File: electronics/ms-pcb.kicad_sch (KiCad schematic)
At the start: 27 parts, among them J1 Left motor, J2 Right motor, J3 XT60-M, U1 ESP32-S3-DEVKITC-1U-N8R2, U2 GY-521

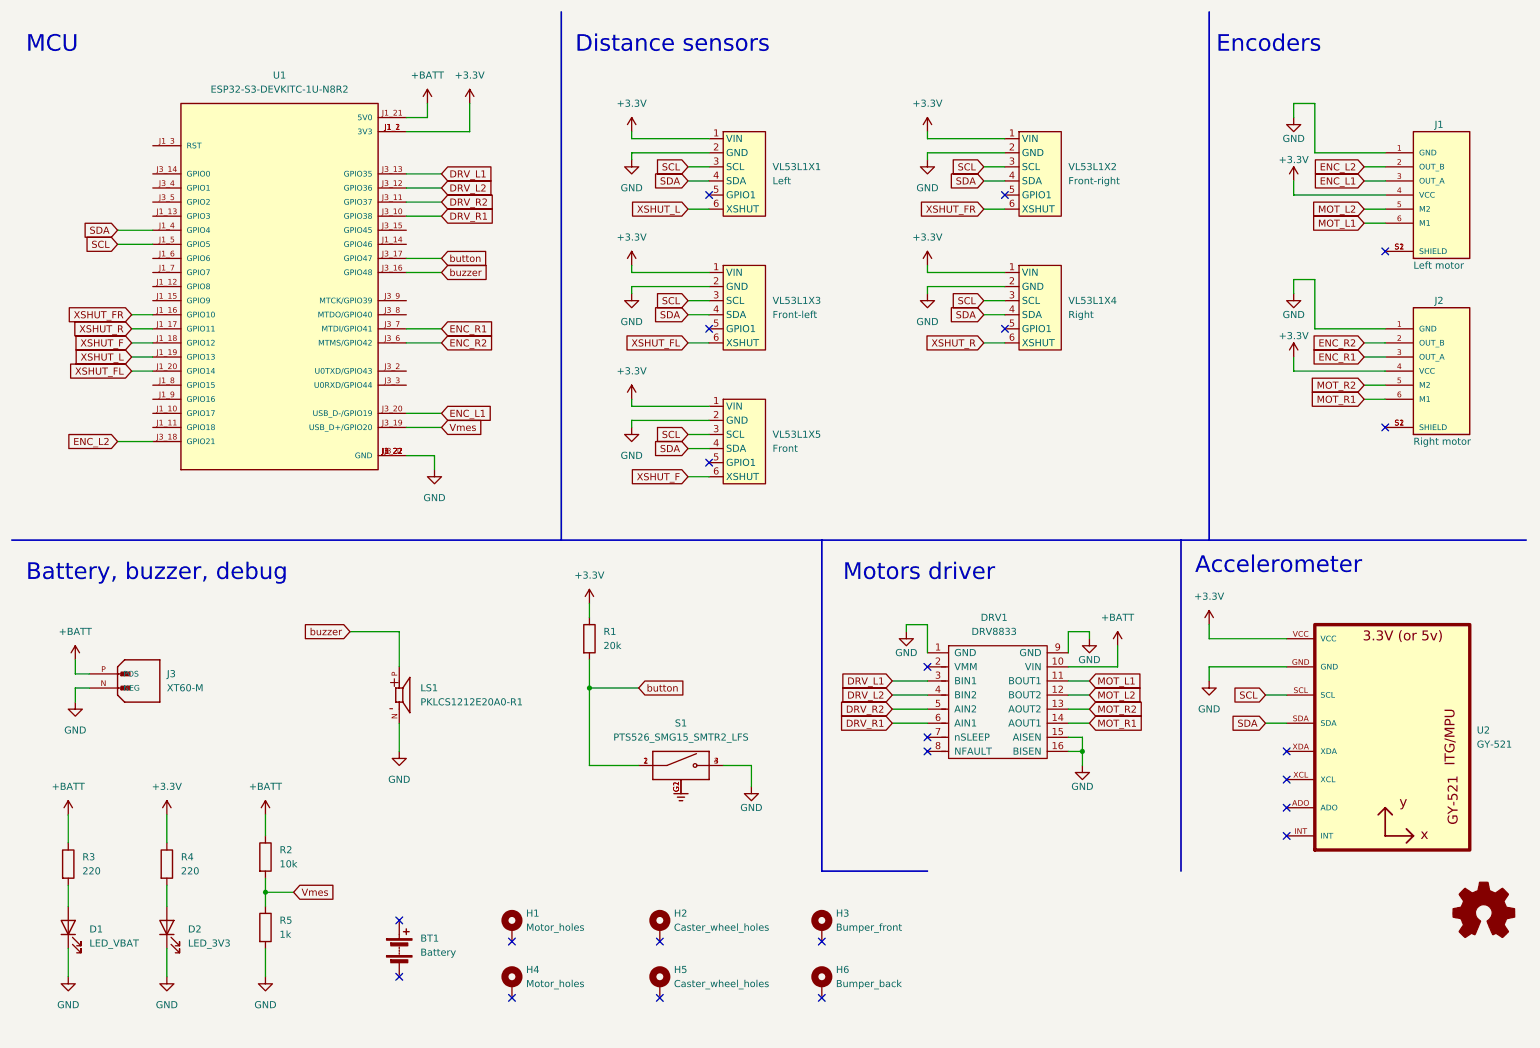
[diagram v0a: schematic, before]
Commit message: elec: start PCB v1.1.0
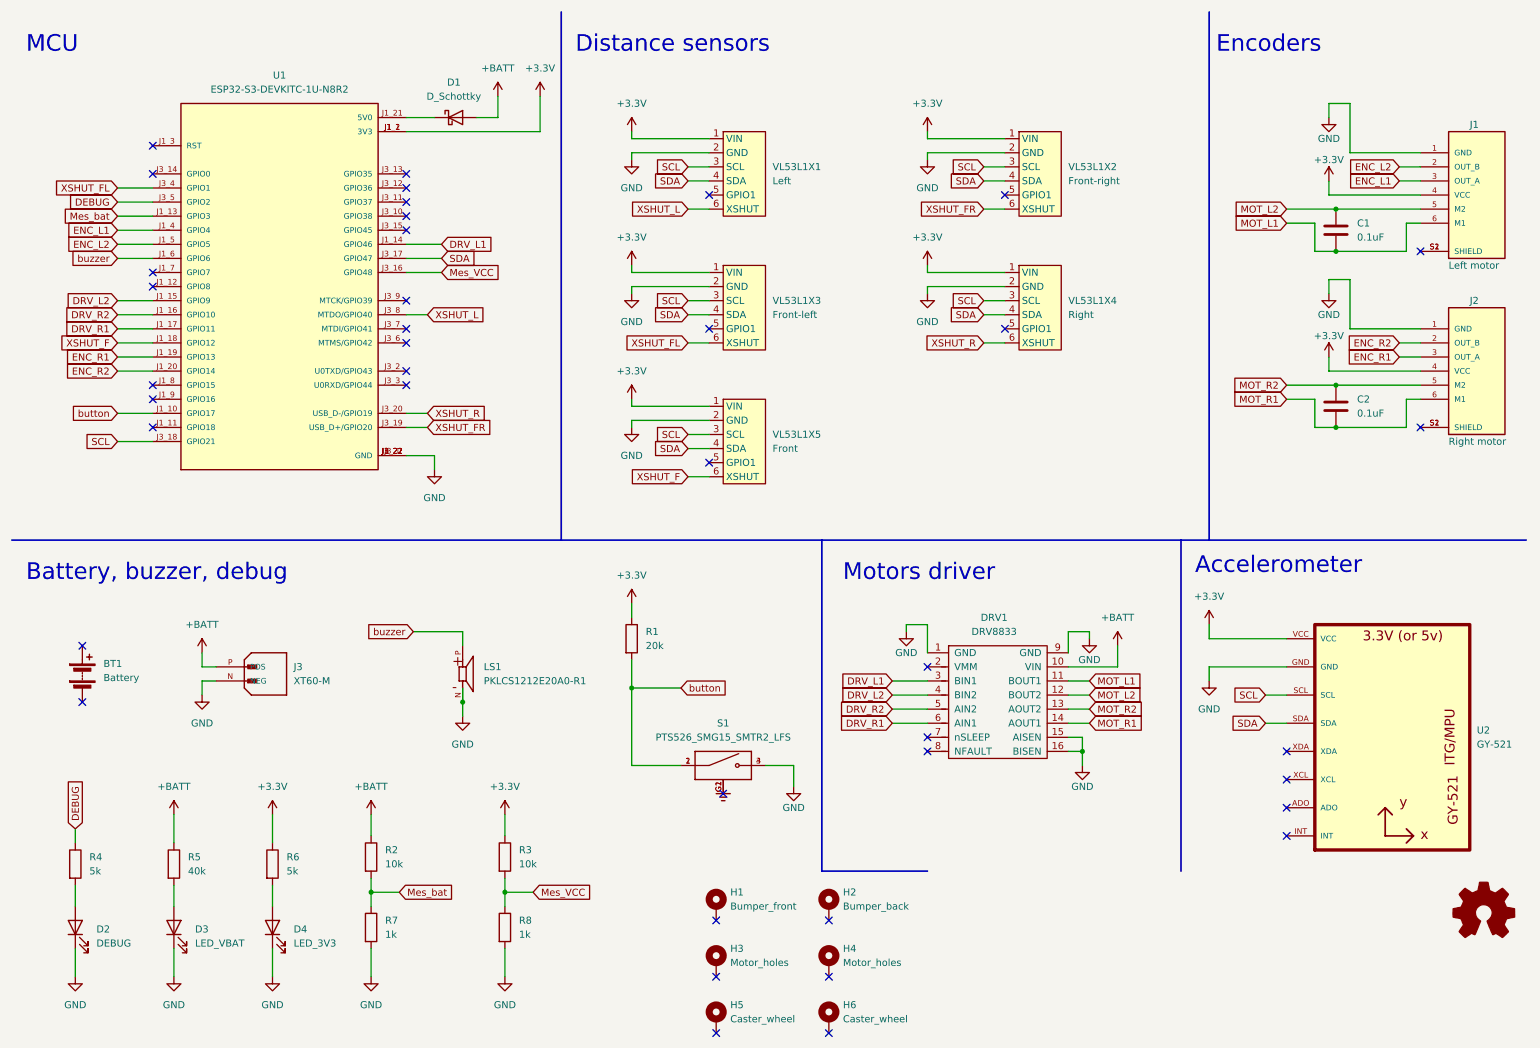
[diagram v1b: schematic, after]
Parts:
- added C1, C2: 0.1uF, Capacitor_THT:CP_Radial_D5.0mm_P2.00mm, symbol Device:C
- added D1: D_Schottky, Diode_SMD:D_1206_3216Metric_Pad1.42x1.75mm_HandSolder, symbol Device:D_Schottky
- added D2: DEBUG, LED_SMD:LED_1206_3216Metric_Pad1.42x1.75mm_HandSolder, symbol Device:LED
- added R3: 10k, Resistor_SMD:R_1206_3216Metric_Pad1.30x1.75mm_HandSolder, symbol Device:R
- added R4: 5k, Resistor_SMD:R_1206_3216Metric_Pad1.30x1.75mm_HandSolder, symbol Device:R
- added R8: 1k, Resistor_SMD:R_1206_3216Metric_Pad1.30x1.75mm_HandSolder, symbol Device:R
- H5: renamed from H2; value Caster_wheel_holes -> Caster_wheel
- H6: renamed from H5; value Caster_wheel_holes -> Caster_wheel
- J3: Description_1 (none) -> Plug; DC supply; XT60; male; PIN: 2; for cable; soldered; 3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
- R5: renamed from R3; value 220 -> 40k
- R6: renamed from R4; value 220 -> 5k
- U1: Description_1 (none) -> WiFi Development Tools - 802.11 ESP32-S3 Gen-Purpose Dev Bd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
- U2: Description_1 (none) -> Triple Axis Accelerometer Gyro Breakout
- renumbered D1 to D3, D2 to D4, H3 to H1, H6 to H2, H1 to H3, R5 to R7
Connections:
- net +3.3V: now also R3.1
- net +BATT: now also D1.2 (A); no longer U1.J1_21 (5V0)
- net DRV_L1: now also U1.J1_14 (GPIO46); no longer U1.J3_13 (GPIO35)
- net DRV_L2: now also U1.J1_15 (GPIO9); no longer U1.J3_12 (GPIO36)
- net DRV_R1: now also U1.J1_17 (GPIO11); no longer U1.J3_10 (GPIO38)
- net DRV_R2: now also U1.J1_16 (GPIO10); no longer U1.J3_11 (GPIO37)
- net ENC_L1: now also U1.J1_4 (GPIO4); no longer U1.J3_20 (USB_D-/GPIO19)
- net ENC_L2: now also U1.J1_5 (GPIO5); no longer U1.J3_18 (GPIO21)
- net ENC_R1: now also U1.J1_19 (GPIO13); no longer U1.J3_7 (MTDI/GPIO41)
- net ENC_R2: now also U1.J1_20 (GPIO14); no longer U1.J3_6 (MTMS/GPIO42)
- net GND: now also D2.1 (K), R8.2
- net MOT_L1: now also C1.2
- net MOT_L2: now also C1.1
- net MOT_R1: now also C2.2
- net MOT_R2: now also C2.1
- net SCL: now also U1.J3_18 (GPIO21); no longer U1.J1_5 (GPIO5)
- net SDA: now also U1.J3_17 (GPIO47); no longer U1.J1_4 (GPIO4)
- net XSHUT_FL: now also U1.J3_4 (GPIO1); no longer U1.J1_20 (GPIO14)
- net XSHUT_FR: now also U1.J3_19 (USB_D+/GPIO20); no longer U1.J1_16 (GPIO10)
- net XSHUT_L: now also U1.J3_8 (MTDO/GPIO40); no longer U1.J1_19 (GPIO13)
- net XSHUT_R: now also U1.J3_20 (USB_D-/GPIO19); no longer U1.J1_17 (GPIO11)
- net button: now also U1.J1_10 (GPIO17); no longer U1.J3_17 (GPIO47)
- net buzzer: now also U1.J1_6 (GPIO6); no longer U1.J3_16 (GPIO48)
- net Mes_bat: now reaches U1.J1_13 (GPIO3)
- net Mes_bat: now also R2.2, R7.1
- net DEBUG: now reaches U1.J3_5 (GPIO2)
- net DEBUG: now also R4.1
- removed net Vmes: R2.2, R7.1, U1.J3_19 (USB_D+/GPIO20)
- new net: D2.2 (A), R4.2
- new net: D1.1 (K), U1.J1_21 (5V0)
- new net Mes_VCC: R3.2, R8.1, U1.J3_16 (GPIO48)
- no-connect marks 22 -> 40
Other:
- moved on the sheet: BT1, D3, D4, H1, H2, H3, H4, H5, H6, J1, J2, J3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
